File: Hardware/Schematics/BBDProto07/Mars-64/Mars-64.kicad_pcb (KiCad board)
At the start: 4 copper layers, 50.8 x 50.8 mm, 76 parts, among them J101 Conn_Coaxial, J102 Conn_Coaxial, U101 ADG731, U102 ADG731

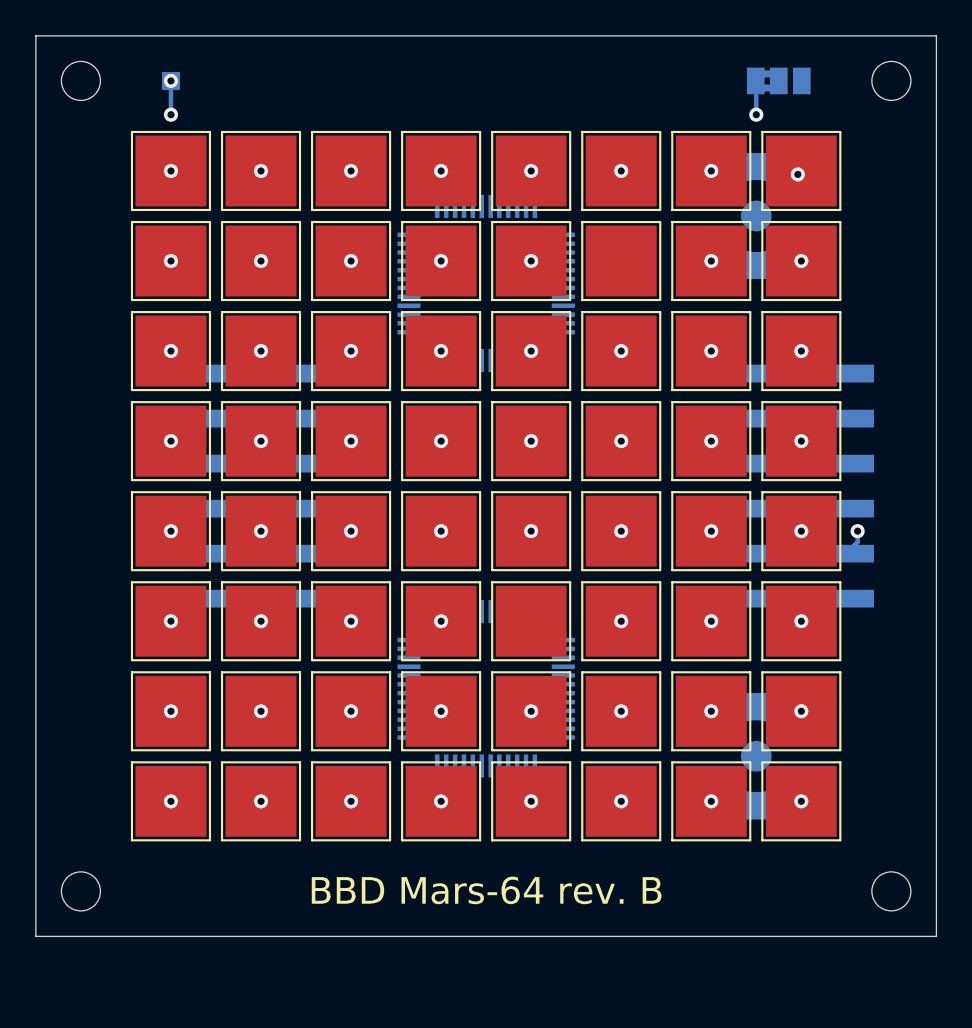
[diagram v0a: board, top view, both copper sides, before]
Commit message: Completed the routing of Mars-64 rev B
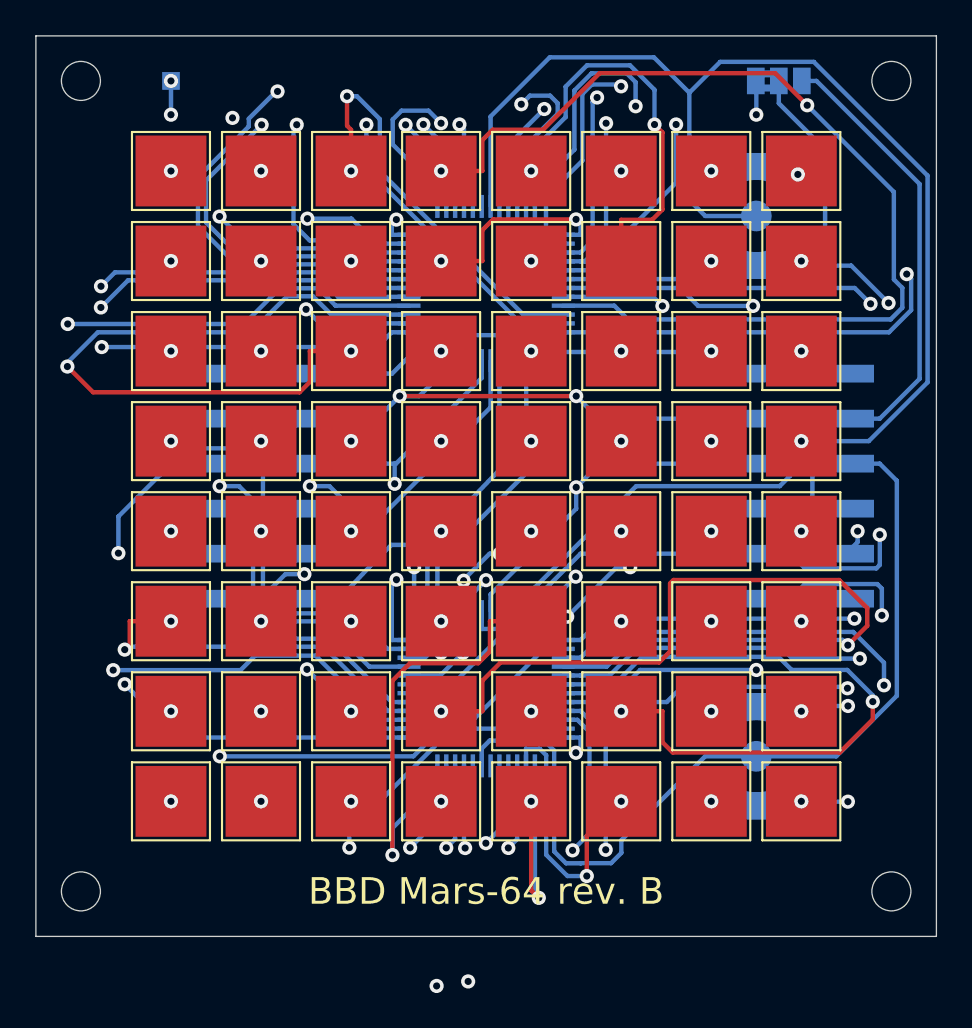
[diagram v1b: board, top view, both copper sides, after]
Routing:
- net GND: track 0.00 -> 89.8 mm, vias 0 -> 2
- net /SPI_MOSI: track 0.00 -> 83.4 mm, vias 0 -> 2
- net Net-(TP101-Pad1): track 0.00 -> 72.4 mm, vias 1 -> 2
- net /DA: track 0.00 -> 70.5 mm
- net Net-(TP123-Pad1): track 0.00 -> 69.1 mm, vias 1 -> 2
- net Net-(TP219-Pad1): track 0.00 -> 66.1 mm, vias 1 -> 2
- net Net-(TP122-Pad1): track 0.00 -> 65.0 mm, vias 1 -> 2
- net /~SPI_CE: track 0.00 -> 64.2 mm, vias 0 -> 2
- net Net-(J101-Pad2): track 0.00 -> 64.1 mm, vias 0 -> 3
- net Net-(TP217-Pad1): track 0.00 -> 60.4 mm, vias 1 -> 2
- net Net-(TP120-Pad1): track 0.00 -> 59.8 mm, vias 1 -> 2
- net /VCC3V3: track 0.00 -> 58.3 mm
- net Net-(TP104-Pad1): track 0.00 -> 58.1 mm, vias 1 -> 2
- net Net-(TP124-Pad1): track 0.00 -> 57.0 mm, vias 1 -> 2
- net Net-(TP121-Pad1): track 0.00 -> 53.5 mm, vias 1 -> 2
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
